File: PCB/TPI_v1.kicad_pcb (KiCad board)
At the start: 2 copper layers, 30 x 65 mm, 20 parts, among them J1 Raspberry pi zero w, J2 BME280, J3 SIG2991, J4 MQ135, J5 Buck, U1 BMI160, U2 DS18B20_1, U3 MCP3008, U4 DS18B20_2, U5 DS18B20_3, U6 DS18B20_4

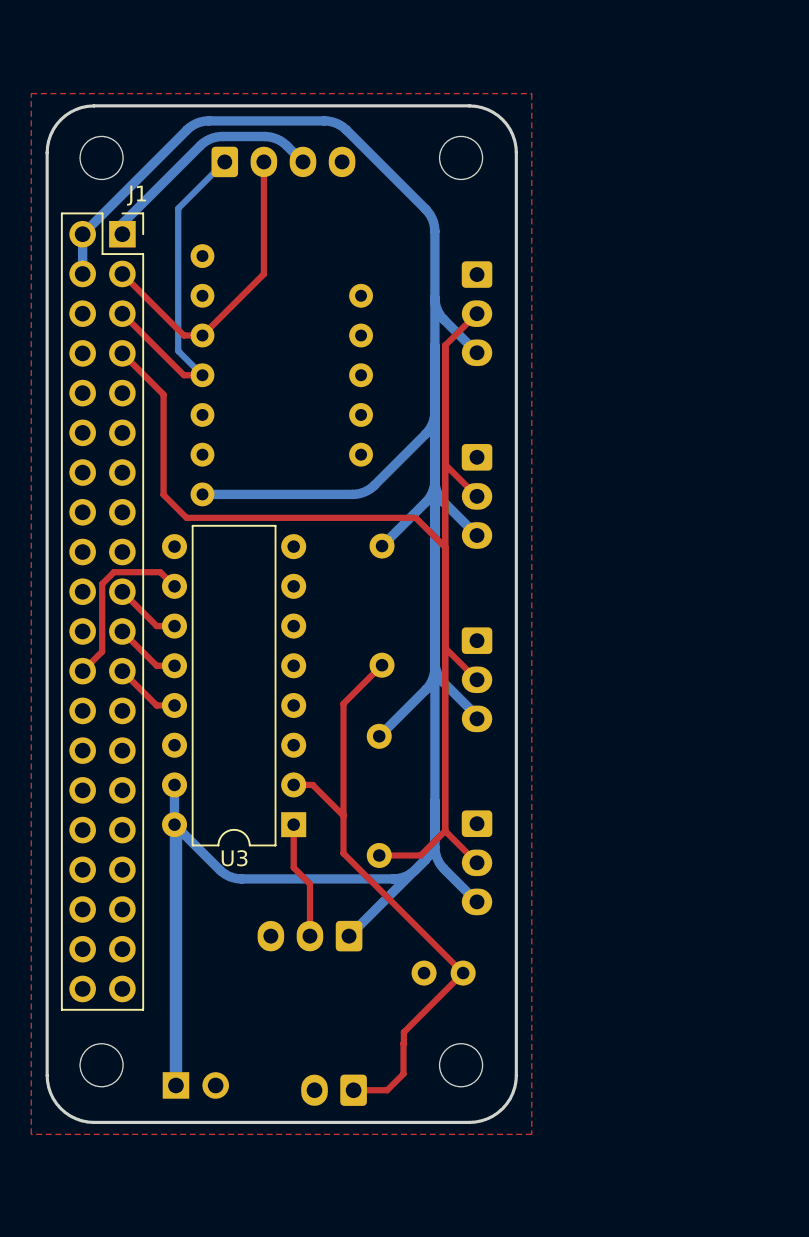
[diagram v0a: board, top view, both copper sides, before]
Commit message: PCB update
V2 PCB
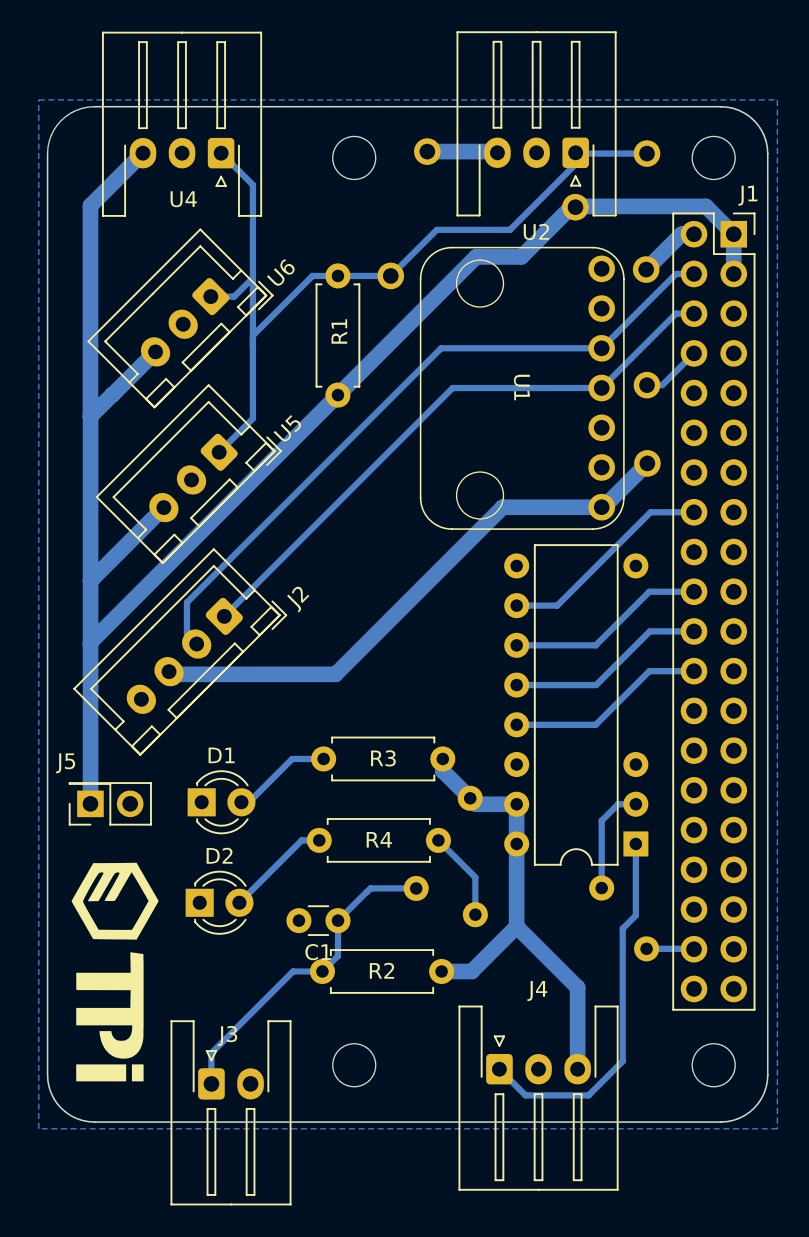
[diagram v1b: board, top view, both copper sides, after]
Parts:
- removed the G*** at (156.5, 86.9)
- added ?: , , F.Cu at (168.1, 99.5)
- added ?: , , F.Cu at (171.6, 93.8)
- added ?: , , F.Cu at (171.9, 101.2)
- added ?: , , F.Cu at (182.9, 72.4)
- added ?: , clipboard:d9ba8ef0-9d5a-486b-8c5f-abd89b3296b6, B.Cu at (160.4, 114.6)
- added ?: , , F.Cu at (180.0, 99.5)
- added ?: , , F.Cu at (182.8, 103.4)
- added ?: , , F.Cu at (182.8, 60.0)
- added ?: , , F.Cu at (166.5, 60.4)
- added ?: , , F.Cu at (182.9, 67.4)
- added ?: , , F.Cu at (182.9, 52.5)
- added ?: , , F.Cu at (178.3, 56.0)
- added ?: , , F.Cu at (168.8, 52.4)
- added D1: LED, LED_THT:LED_D3.0mm, F.Cu at (154.4, 94.0)
- added D2: LED, LED_THT:LED_D3.0mm, F.Cu at (154.3, 100.5)
- added G***: LOGO, Custom:Walle, F.Cu at (148.8, 100.4)
- added R3: 2.2K, Resistor_THT:R_Axial_DIN0207_L6.3mm_D2.5mm_P7.62mm_Horizontal, F.Cu at (169.8, 91.3)
- added R4: 2.2K, Resistor_THT:R_Axial_DIN0207_L6.3mm_D2.5mm_P7.62mm_Horizontal, F.Cu at (169.5, 96.5)
- C1, J3, J5, R1, R2, U1, U4: moved to F.Cu
- J2: footprint Connector_JST:JST_XH_S4B-XH-A-1_1x04_P2.50mm_Horizontal -> Connector_JST:JST_XH_B4B-XH-A_1x04_P2.50mm_Vertical; moved to F.Cu
- J4: footprint Connector_JST:JST_XH_B3B-XH-A_1x03_P2.50mm_Vertical -> Connector_JST:JST_XH_S3B-XH-A-1_1x03_P2.50mm_Horizontal; moved to F.Cu
- U2: value DS18B20_1 -> DS18B20_2; moved to F.Cu
- U5: value DS18B20_3 -> DS18B20_2; footprint Connector_JST:JST_XH_S3B-XH-A-1_1x03_P2.50mm_Horizontal -> Connector_JST:JST_XH_B3B-XH-A_1x03_P2.50mm_Vertical; moved to F.Cu
- U6: value DS18B20_4 -> DS18B20_2; footprint Connector_JST:JST_XH_S3B-XH-A-1_1x03_P2.50mm_Horizontal -> Connector_JST:JST_XH_B3B-XH-A_1x03_P2.50mm_Vertical; moved to F.Cu
- moved J1 39.1 mm to (185.8, 57.7)
- moved U6 37.8 mm to (155.0, 61.7), turned to -135 degrees
- moved U2 31.8 mm to (178.3, 52.5), turned to 180 degrees
- moved J2 29.1 mm to (155.8, 82.1), turned to -135 degrees
- moved R2 27.5 mm to (169.7, 104.8), turned to 180 degrees
- moved U4 25.4 mm to (155.6, 52.5), turned to 180 degrees
- moved R1 22.0 mm to (163.1, 68.0), turned to 90 degrees
- moved U3 21.9 mm to (182.1, 96.7)
- moved U5 20.0 mm to (155.5, 71.7), turned to -135 degrees
- moved J5 18.8 mm to (147.3, 94.1)
- moved ? 16.2 mm to (187.1, 110.8)
- moved ? 16.2 mm to (164.1, 110.8)
- moved ? 16.2 mm to (187.1, 52.8)
- moved ? 16.2 mm to (164.1, 52.8)
- moved U1 15.4 mm to (174.9, 67.6)
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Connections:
- J1 pad 15: unconnected-(J1-GPIO22-Pad15) -> ~{CS}
- J1 pad 17: unconnected-(J1-3.3V-Pad17) -> +3.3V
- J1 pad 24: ~{CS} -> unconnected-(J1-GPIO8-Pad24)
- J1 pad 37: unconnected-(J1-GPIO26-Pad37) -> Server
- J4 pad 1: +5V -> ADC0
- J4 pad 2: ADC0 -> GND
- J4 pad 3: GND -> +5V
- U1 pad 1: +5V -> +3.3V
- U2 pad 1: GND -> DQ
- U2 pad 2: DQ -> GND
- U4 pad 1: GND -> DQ
- U4 pad 2: DQ -> GND
- U5 pad 1: GND -> DQ
- U5 pad 2: DQ -> GND
- U6 pad 1: GND -> DQ
- U6 pad 2: DQ -> GND
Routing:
- net DQ: track 122.0 -> 59.2 mm
- net +5V: track 208.7 -> 147.0 mm
- net SDA: track 19.5 -> 44.0 mm
- net +3.3V: track 16.8 -> 40.2 mm
- net ADC0: track 7.56 -> 23.7 mm
- net SCL: track 22.5 -> 38.0 mm
- net ADC1: track 39.5 -> 27.7 mm
- net Server: track 0.00 -> 9.34 mm
- net SCLK: track 4.24 -> 12.8 mm
- net MOSI: track 4.24 -> 12.8 mm
- net MISO: track 4.24 -> 12.8 mm
- net Net-(D2-A): track 0.00 -> 6.76 mm
- net Net-(D1-A): track 0.00 -> 6.40 mm
- net ~{CS}: track 11.4 -> 13.8 mm
- added copper zone on B.Cu, net GND
- removed copper zone on F.Cu, net GND
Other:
- board size 30 x 65 mm -> 46.1 x 64.9 mm
